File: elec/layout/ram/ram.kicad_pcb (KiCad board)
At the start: 2 copper layers, 40 x 40 mm, 56 parts, among them U1 _NXP_Semicon_MIMX8MM6CVTKZAA

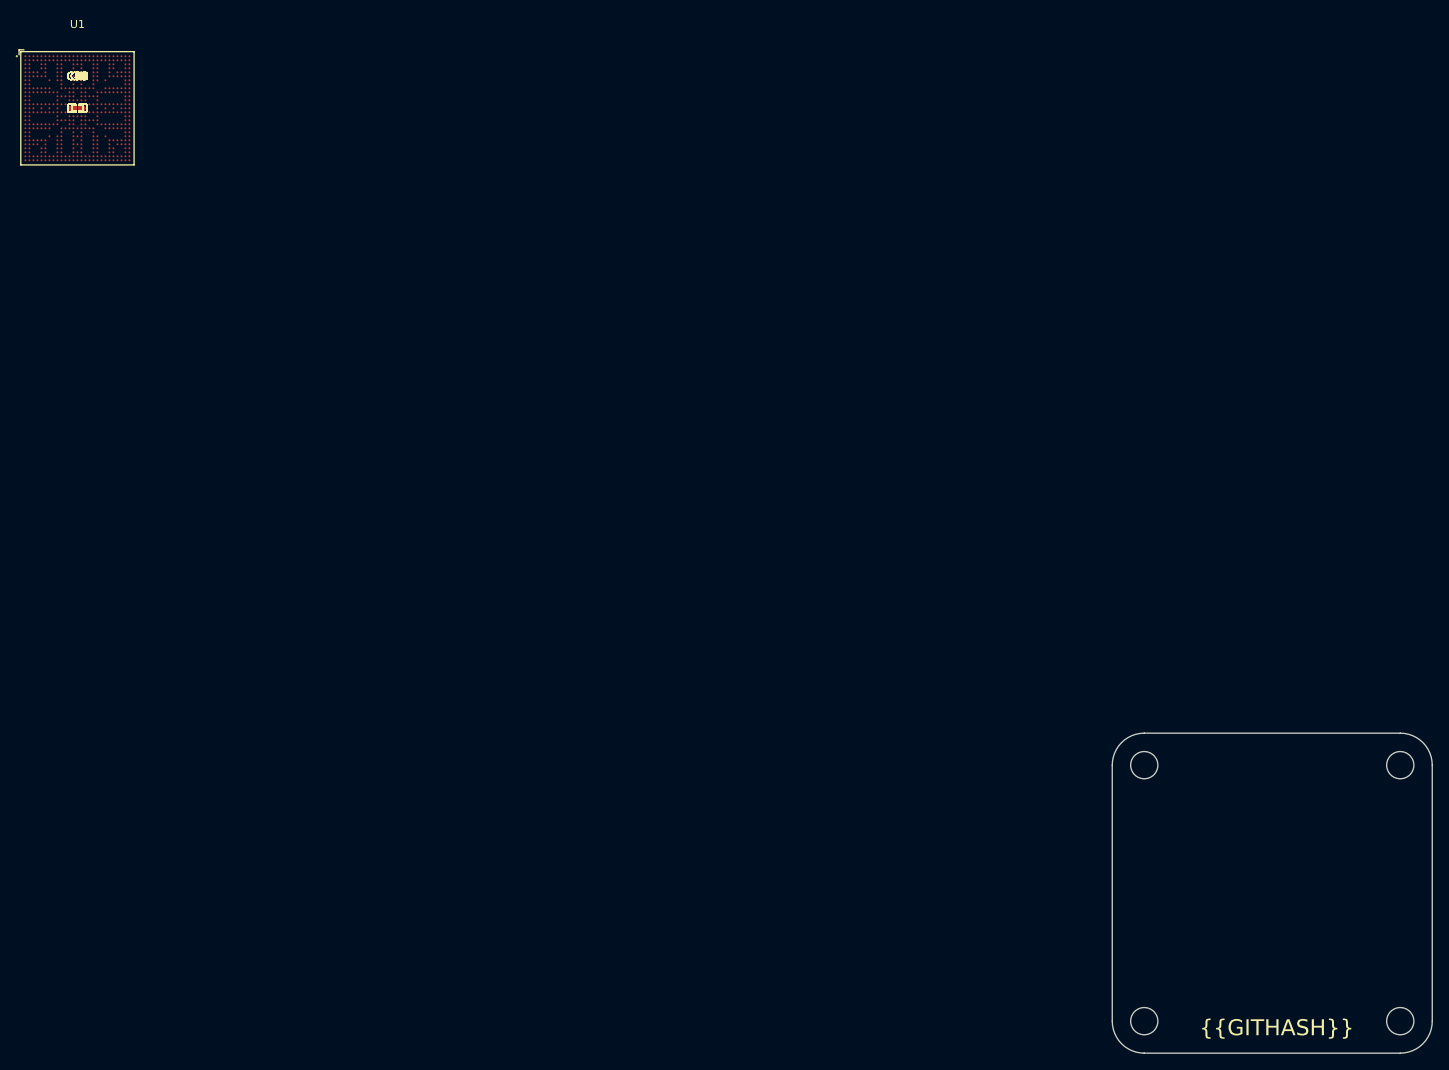
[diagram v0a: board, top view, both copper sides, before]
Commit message: Building! started on layout
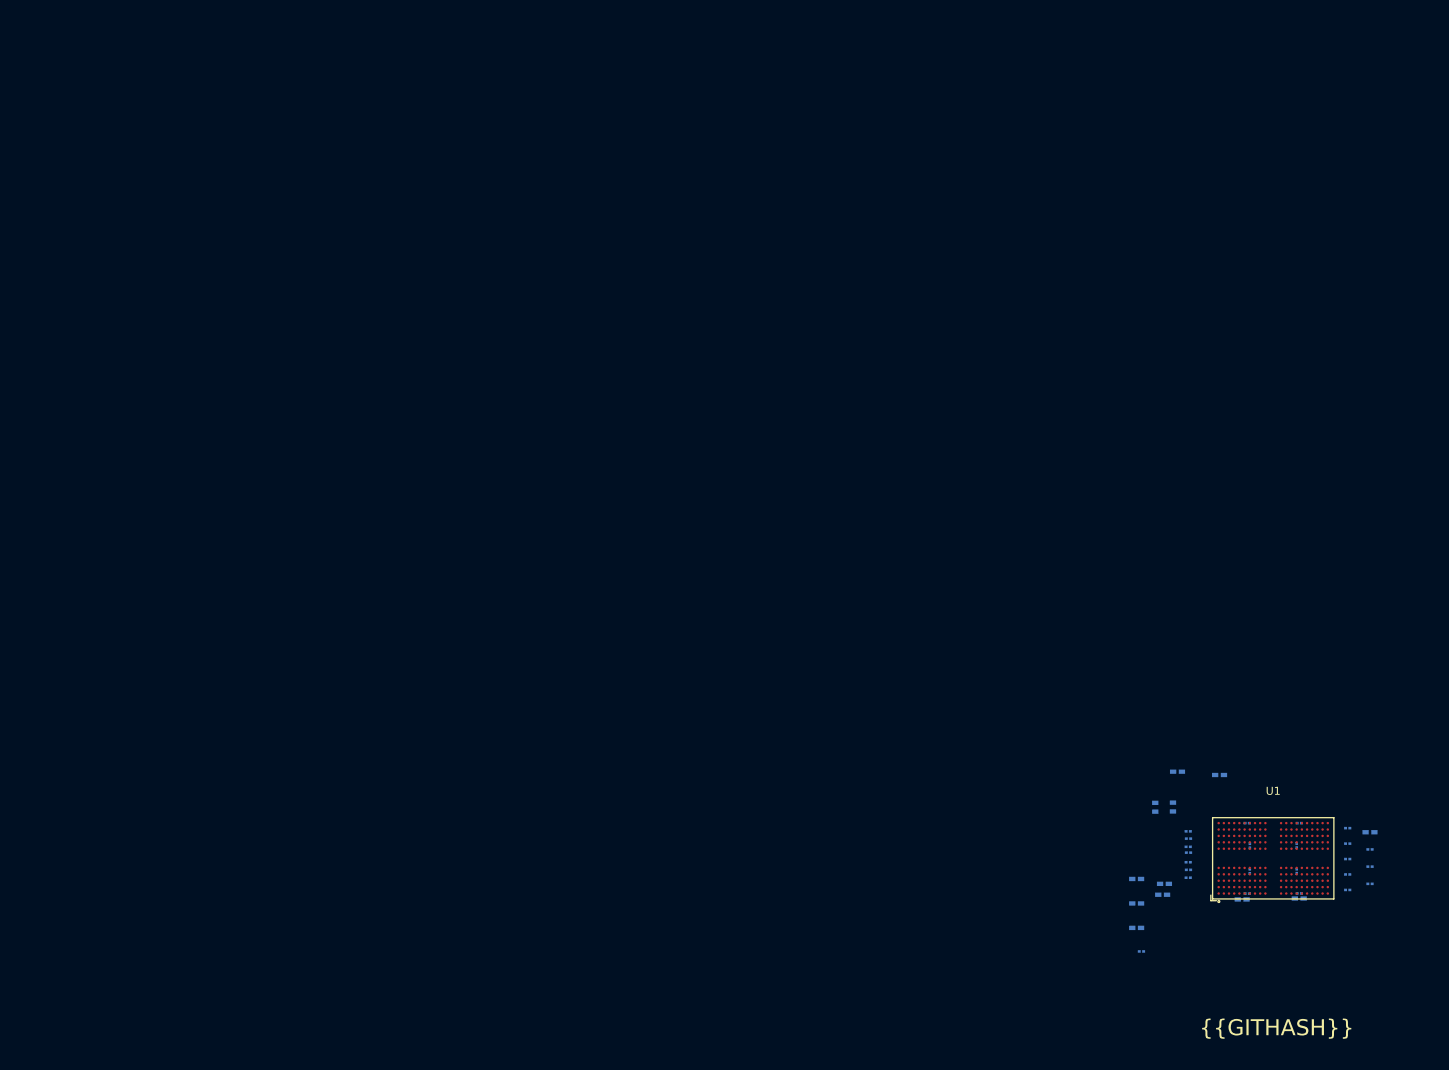
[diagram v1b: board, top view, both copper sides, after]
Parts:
- removed C37, C48: 10µF ±20% 6.3V X5R, lcsc:C0402
- removed C38, C39, C40, C41, C42, C43, C50, C51, C52, C53, C54: 1µF ±20% 6.3V X5R, lcsc:C0201
- removed C44, C46, C47, C55: 220nF ±20% 6.3V X5R, lcsc:C0201
- removed C45: 2.2µF ±20% 6.3V X5R, lcsc:C0402
- removed C49: 4.7µF ±20% 10V X5R, lcsc:C0402
- C1: value 2.2µF ±20% 6.3V X5R -> 10µF ±20% 6.3V X5R; footprint lcsc:C0201 -> lcsc:C0402; moved to B.Cu
- C10, C11, C13, C16, C17, C24, C26, C27, C28, C30: moved to B.Cu
- C12, C14, C32, C33, C34, C35, C4, C5, C6, C7, C8, C9: value 1µF ±20% 6.3V X5R -> 220nF ±20% 6.3V X5R; moved to B.Cu
- C15, C2, C3, C36: value 10µF ±20% 6.3V X5R -> 220nF ±20% 6.3V X5R; footprint lcsc:C0402 -> lcsc:C0201; moved to B.Cu
- C18, C19, C20, C21, C22, C23, C29: value 220nF ±20% 6.3V X5R -> 10µF ±20% 6.3V X5R; footprint lcsc:C0201 -> lcsc:C0402; moved to B.Cu
- C25: value 4.7µF ±20% 10V X5R -> 10µF ±20% 6.3V X5R; moved to B.Cu
- C31: value 1µF ±20% 6.3V X5R -> 10µF ±20% 6.3V X5R; footprint lcsc:C0201 -> lcsc:C0402; moved to B.Cu
- U1: value _NXP_Semicon_MIMX8MM6CVTKZAA -> _SK_HYNIX_H9HCNNNBKUMLXR_NEE; footprint lcsc:BGA-486_L14.0-W14.0-P0.50-TL_NXP_MIMX8MMXDVTLZXA -> lcsc:FBGA-200_L15.0-W10.0-BL_H9HCNNNBKUMLXR
- moved C13 188.4 mm to (161.6, 96.9)
- moved C12 187.3 mm to (161.6, 94.8)
- moved C6 186.4 mm to (158.8, 97.7), turned to 180 degrees
- moved C11 186.2 mm to (161.6, 92.6)
- moved C5 185.4 mm to (158.8, 95.8), turned to 180 degrees
- moved C1 185.2 mm to (161.6, 90.5), turned to 180 degrees
- moved C4 184.4 mm to (158.8, 93.8), turned to 180 degrees
- moved C3 183.5 mm to (158.8, 91.9), turned to 180 degrees
- moved C2 182.5 mm to (158.8, 90.0), turned to 180 degrees
- moved C20 181.9 mm to (152.7, 98.8), turned to 180 degrees
- moved C27 181.5 mm to (152.7, 98.1), turned to 180 degrees
- moved C24 179.8 mm to (152.4, 95.4), turned to 90 degrees
- moved C26 178.1 mm to (152.4, 92.2), turned to -90 degrees
- moved C35 177.0 mm to (152.7, 89.4), turned to 180 degrees
- moved U1 176.4 mm to (149.5, 93.8)
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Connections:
- net dram_ac00 renamed signal-16
- net dram_ac03 renamed signal-14
- net dram_ac10 renamed signal-49
- net dram_ac23 renamed signal-25
- net dram_ac24 renamed signal-55
- net dram_ac32 renamed signal-28
- net dram_alert_n renamed signal-12
- net dram_dq00 renamed zq0
- net dram_dq07 renamed signal-53
- net dram_dq08 renamed signal-3
- net dram_dq11 renamed signal-0
- net dram_dq15 renamed signal-33
- net dram_dq17 renamed signal-5
- net dram_dq20 renamed signal-9
- net dram_dqs0_n renamed signal-34
- net dram_zn renamed signal-59
- net i2c1_scl renamed signal-24
- net i2c1_sda renamed signal-36
- net i2c2_scl renamed signal-57
- net i2c3_scl renamed signal-11
- net mipi_dsi_clk_p renamed signal-22
- net mipi_dsi_d0_p renamed signal-26
- net vdd_dram_pll_0p8 renamed ck_cb
- C1 pad 1: *BC98.processor-net-1 -> NVCC_DRAM_1V1
- C10 pad 1: NVCC_ENET -> NVCC_DRAM_1V1
- C11 pad 1: NVCC_SD2 -> NVCC_DRAM_1V1
- C12 pad 1: *BC98.processor-net-0 -> NVCC_DRAM_1V1
- C13 pad 1: VDDA_1V8 -> NVCC_DRAM_1V1
- C14 pad 1: VDDA_1V8 -> NVCC_DRAM_1V1
- C15 pad 1: VDDA_1V8 -> NVCC_DRAM_1V1
- C16 pad 1: VDDA_1V8 -> NVCC_DRAM_1V1
- C17 pad 1: VDDA_1V8 -> NVCC_DRAM_1V1
- C18 pad 1: VDDA_1V8 -> NVCC_DRAM_1V1
- C19 pad 1: VDDA_1V8 -> NVCC_DRAM_1V1
- C20 pad 1: VDDA_1V8 -> NVCC_DRAM_1V1
- C21 pad 1: VDDA_1V8 -> NVCC_DRAM_1V1
- C22 pad 1: VDDA_1V8 -> NVCC_DRAM_1V1
- C23 pad 1: VDDA_1V8 -> NVCC_DRAM_1V1
- C24 pad 1: VDDA_1V8 -> NVCC_DRAM_1V1
- C25 pad 1: VDD_3V3 -> VDD_1V8
- C26 pad 1: VDD_3V3 -> VDD_1V8
- C27 pad 1: VDD_3V3 -> VDD_1V8
- C28 pad 1: VDD_3V3 -> VDD_1V8
- C29 pad 1: VDD_3V3 -> VDD_1V8
- C30 pad 1: VDD_ARM_0V9 -> VDD_1V8
- C31 pad 1: VDD_ARM_0V9 -> VDD_1V8
- C32 pad 1: VDD_ARM_0V9 -> VDD_1V8
- C33 pad 1: VDD_ARM_0V9 -> VDD_1V8
- C34 pad 1: VDD_ARM_0V9 -> VDD_1V8
- C35 pad 1: VDD_ARM_0V9 -> VDD_1V8
- C36 pad 1: VDD_DRAM_0V9 -> VDD_1V8
- U1 pad A1: GND -> *5FE8.RAM.RAM-net-0
- U1 pad A10: mipi_dsi_d1_n -> GND
- U1 pad A11: mipi_dsi_clk_n -> *5FE8.RAM.RAM-net-0
- U1 pad A12: mipi_dsi_d2_n -> *5FE8.RAM.RAM-net-0
- U1 pad A2: dram_dqs0_p -> *5FE8.RAM.RAM-net-0
- U1 pad A3: dram_dq06 -> GND
- U1 pad A4: dram_dm0 -> NVCC_DRAM_1V1
- U1 pad A8: ecspi2_miso -> *5FE8.RAM.RAM-net-1
- U1 pad A9: mipi_dsi_d0_n -> NVCC_DRAM_1V1
- U1 pad AA1: dram_dqs2_p -> *5FE8.RAM.RAM-net-0
- U1 pad AA10: GND -> NVCC_DRAM_1V1
- U1 pad AA9: GND -> signal-42
- U1 pad AB1: dram_dm2 -> *5FE8.RAM.RAM-net-0
- U1 pad AB10: gpio1_io12 -> GND
- U1 pad AB2: dram_dq16 -> *5FE8.RAM.RAM-net-0
- U1 pad AB4: dram_ac20 -> NVCC_DRAM_1V1
- U1 pad AB5: dram_ac21 -> GND
- U1 pad AB9: gpio1_io15 -> NVCC_DRAM_1V1
- U1 pad B1: dram_dq05 -> *5FE8.RAM.RAM-net-0
- U1 pad B10: mipi_dsi_d1_p -> NVCC_DRAM_1V1
- U1 pad B12: mipi_dsi_d2_p -> *5FE8.RAM.RAM-net-0
- U1 pad B3: GND -> NVCC_DRAM_1V1
- U1 pad B5: dram_dq01 -> NVCC_DRAM_1V1
- U1 pad B8: ecspi2_mosi -> NVCC_DRAM_1V1
- U1 pad C1: dram_dq04 -> GND
- U1 pad C10: GND -> signal-38
- U1 pad C2: GND -> signal-4
- U1 pad C9: GND -> signal-39
- U1 pad D1: dram_dq03 -> NVCC_DRAM_1V1
- U1 pad D2: dram_dq02 -> GND
- U1 pad D5: dram_ac11 -> NVCC_DRAM_1V1
- U1 pad D9: i2c2_sda -> GND
- U1 pad E1: dram_dq14 -> GND
- U1 pad E3: GND -> signal-40
- U1 pad F1: dram_dm1 -> VDD_1V8
- U1 pad F10: i2c3_sda -> NVCC_DRAM_1V1
- U1 pad F3: GND -> NVCC_DRAM_1V1
- U1 pad F5: dram_ac01 -> NVCC_DRAM_1V1
- U1 pad G1: dram_dqs1_p -> GND
- U1 pad G2: dram_dq09 -> NVCC_DRAM_1V1
- U1 pad G9: GND -> VDD_1V8
- U1 pad H1: dram_dqs1_n -> NVCC_DRAM_1V1
- U1 pad H10: VDD_3V3 -> signal-7
- U1 pad H2: GND -> signal-31
- U1 pad J1: dram_dq10 -> GND
- U1 pad J10: VDD_DRAM_0V9 -> GND
- U1 pad J11: VDDA_1V8 -> signal-43
- U1 pad J12: VDDA_1V8 -> GND
- U1 pad J5: dram_ac07 -> *5FE8.RAM.RAM-net-1
- U1 pad K1: dram_dq13 -> NVCC_DRAM_1V1
- U1 pad K12: VDD_DRAM_0V9 -> NVCC_DRAM_1V1
- U1 pad K2: dram_dq12 -> GND
- U1 pad K3: GND -> NVCC_DRAM_1V1
- U1 pad K4: dram_ac02 -> GND
- U1 pad K5: dram_ac14 -> *5FE8.RAM.RAM-net-1
- U1 pad K8: NVCC_DRAM_1V1 -> *5FE8.RAM.RAM-net-1
- U1 pad K9: NVCC_DRAM_1V1 -> GND
- U1 pad N1: dram_ac26 -> NVCC_DRAM_1V1
- U1 pad N10: VDD_DRAM_0V9 -> NVCC_DRAM_1V1
- U1 pad N11: VDD_DRAM_0V9 -> GND
- U1 pad N12: GND -> NVCC_DRAM_1V1
- U1 pad N2: dram_ac19 -> GND
- U1 pad N3: GND -> NVCC_DRAM_1V1
- U1 pad N4: dram_ac12 -> GND
- U1 pad N5: dram_ac13 -> *5FE8.RAM.RAM-net-1
- U1 pad N8: NVCC_DRAM_1V1 -> *5FE8.RAM.RAM-net-1
- U1 pad N9: NVCC_DRAM_1V1 -> GND
- U1 pad P1: dram_vref -> GND
- U1 pad P12: VDD_DRAM_0V9 -> GND
- U1 pad P5: VDD_DRAM_0V9 -> *5FE8.RAM.RAM-net-1
- U1 pad R1: dram_reset_n -> NVCC_DRAM_1V1
- U1 pad R10: VDD_DRAM_0V9 -> signal-50
- U1 pad R11: VDD_DRAM_0V9 -> signal-58
- U1 pad R12: GND -> NVCC_DRAM_1V1
- U1 pad R3: GND -> *5FE8.RAM.RAM-net-1
- U1 pad R5: dram_ac33 -> NVCC_DRAM_1V1
- U1 pad R9: NVCC_DRAM_1V1 -> signal-52
- U1 pad T1: dram_ac234 -> GND
- U1 pad T2: dram_ac35 -> NVCC_DRAM_1V1
- U1 pad T9: NVCC_DRAM_1V1 -> VDD_1V8
- U1 pad U1: dram_ac25 -> VDD_1V8
- U1 pad U10: VDD_DRAM_0V9 -> NVCC_DRAM_1V1
- U1 pad U11: VDD_DRAM_0V9 -> signal-37
- U1 pad U12: GND -> VDD_1V8
- U1 pad U9: NVCC_DRAM_1V1 -> signal-32
- U1 pad V1: dram_dq21 -> GND
- U1 pad V12: VDD_DRAM_0V9 -> GND
- U1 pad V3: GND -> signal-18
- U1 pad V5: dram_ac36 -> GND
- U1 pad V8: NVCC_DRAM_1V1 -> GND
- U1 pad V9: NVCC_DRAM_1V1 -> signal-47
- U1 pad W1: dram_dq18 -> NVCC_DRAM_1V1
- U1 pad W10: VDD_DRAM_0V9 -> signal-15
- U1 pad W11: VDD_DRAM_0V9 -> GND
- U1 pad W12: VDDA_1V8 -> NVCC_DRAM_1V1
- U1 pad W2: dram_dq19 -> GND
- U1 pad W3: GND -> signal-44
- U1 pad W4: dram_ac22 -> GND
- U1 pad W5: dram_ac37 -> NVCC_DRAM_1V1
- U1 pad Y1: dram_dqs2_n -> GND
- U1 pad Y10: VDD_3V3 -> signal-29
- U1 pad Y2: GND -> signal-54
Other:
- board outline removed
